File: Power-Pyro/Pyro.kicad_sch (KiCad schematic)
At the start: 20 parts, among them J1 Conn_01x02, J2 Conn_01x02, J3 Conn_01x02, J4 Conn_01x02, Q1 SSM3J328R, Q2 SSM3J328R, Q3 L2N7002SLLT1G, Q4 L2N7002SLLT1G, Q5 SSM3J328R, Q6 SSM3J328R, Q7 L2N7002SLLT1G, Q8 L2N7002SLLT1G

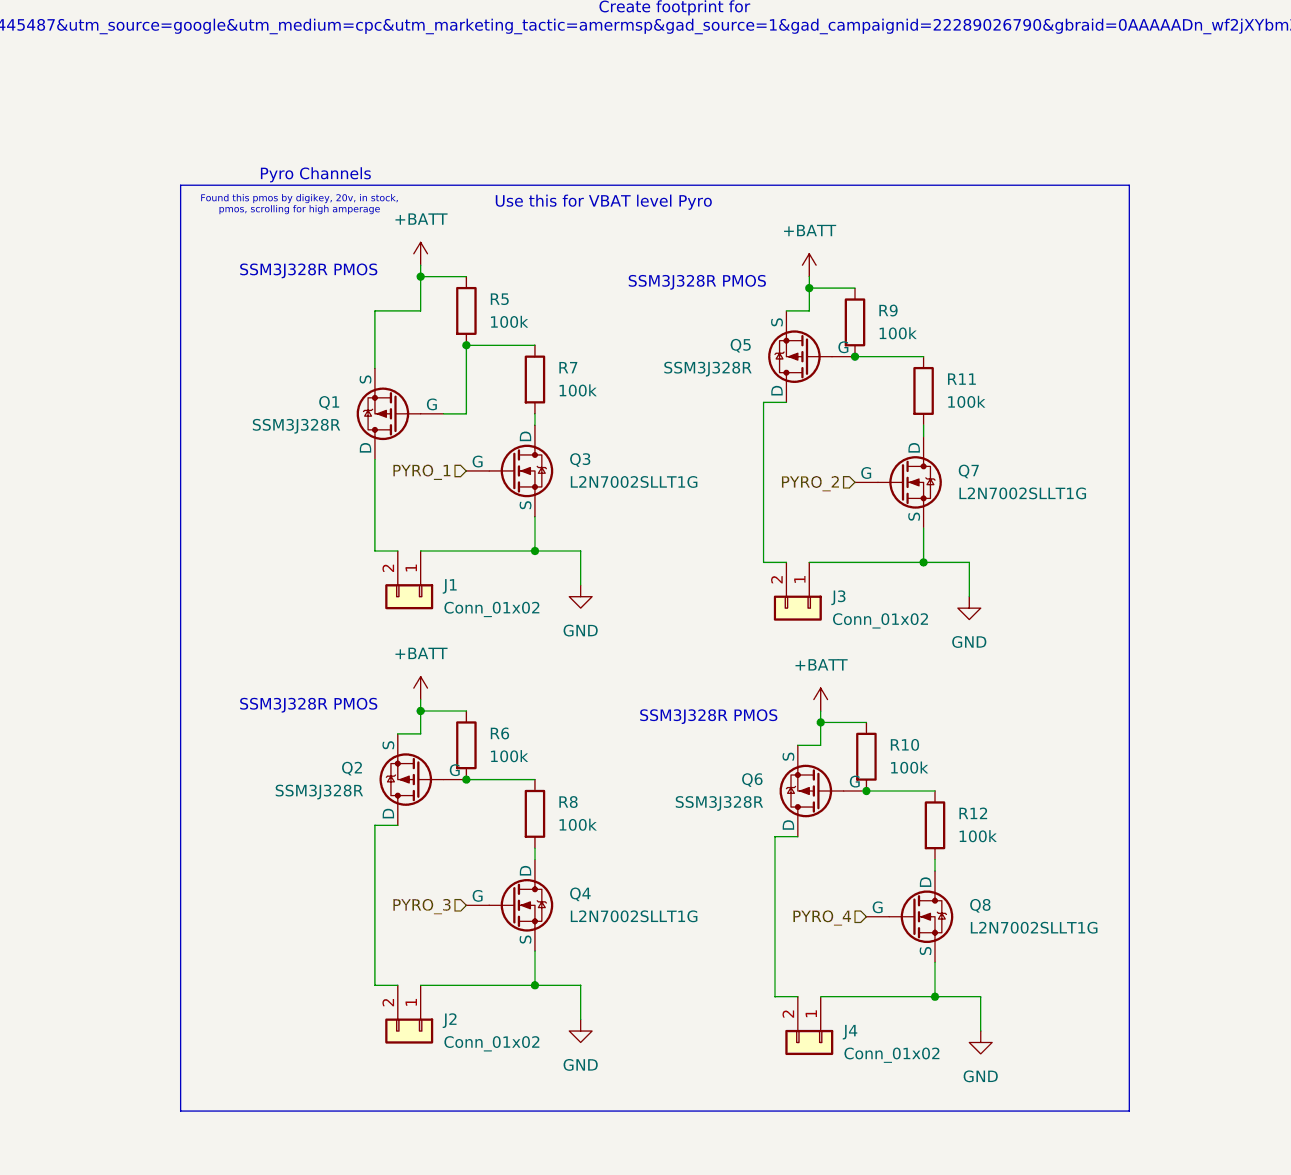
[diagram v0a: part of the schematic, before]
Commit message: 🔌
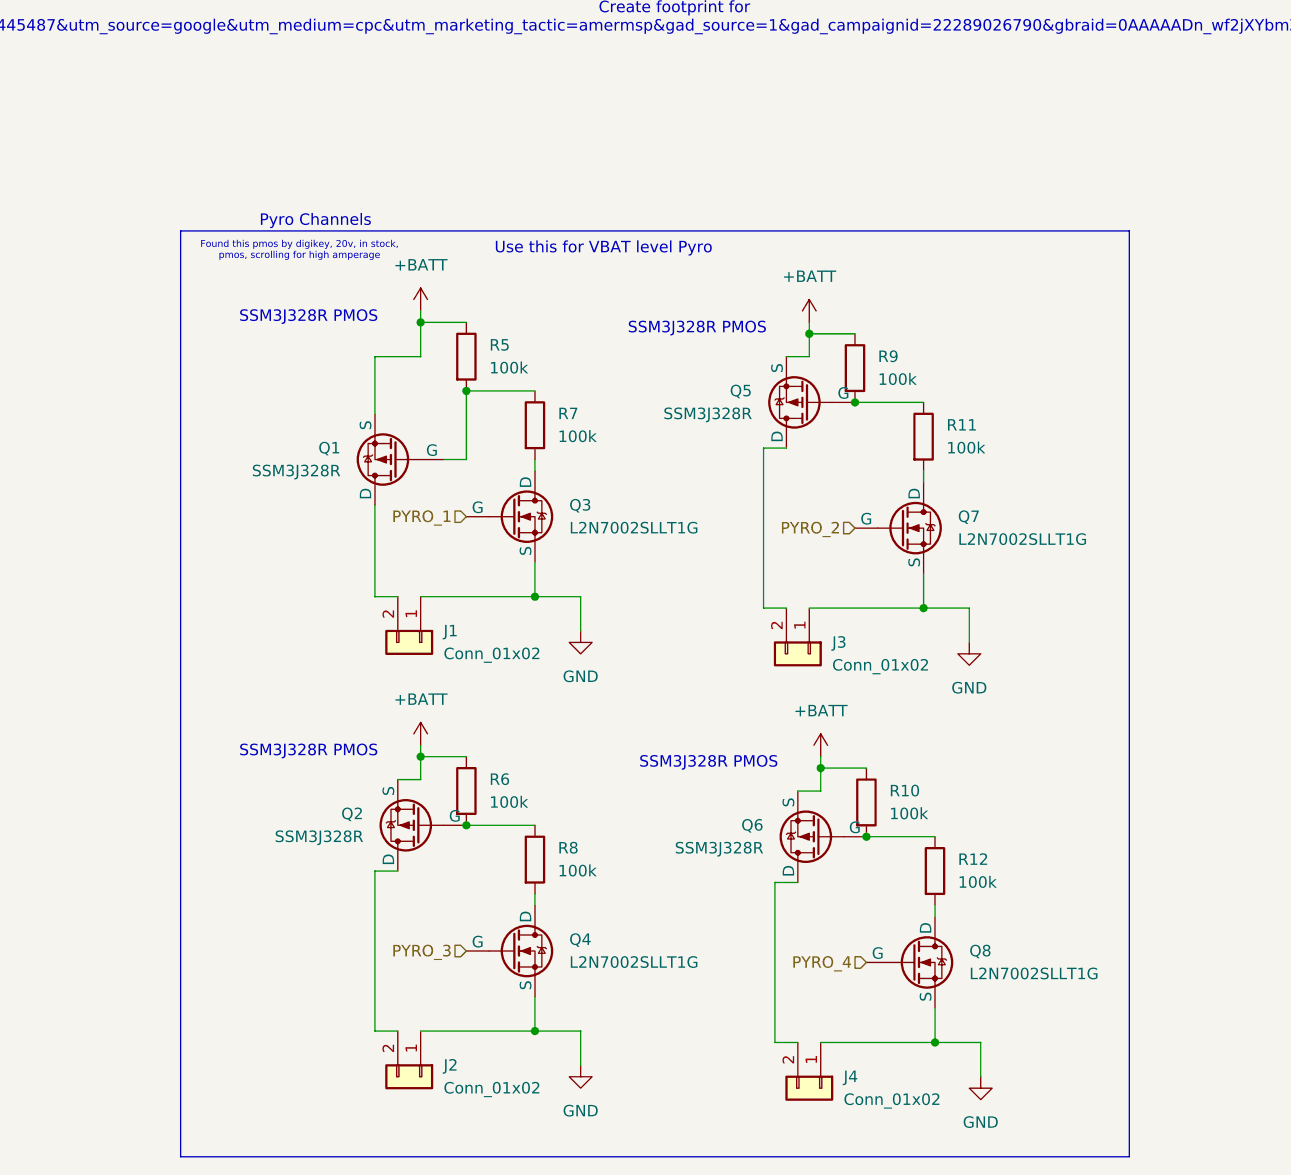
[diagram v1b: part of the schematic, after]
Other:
- moved on the sheet: J1, J2, J3, J4, Q1, Q2, Q3, Q4, Q5, Q6, Q7, Q8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
